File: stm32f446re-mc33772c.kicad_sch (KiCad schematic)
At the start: 43 parts, among them J1 Conn_01x02, J2 USB_B_Micro, J3 Conn_01x03, J4 Conn_01x03, J6 SM06B-GHS-TB, U1 STM32F446RET6, U3 LD1086D2M33TR, U4 AMS1117-3.3, U6 LMR51450SDRRR, U7 SN65HVD232, Y1 16MHz

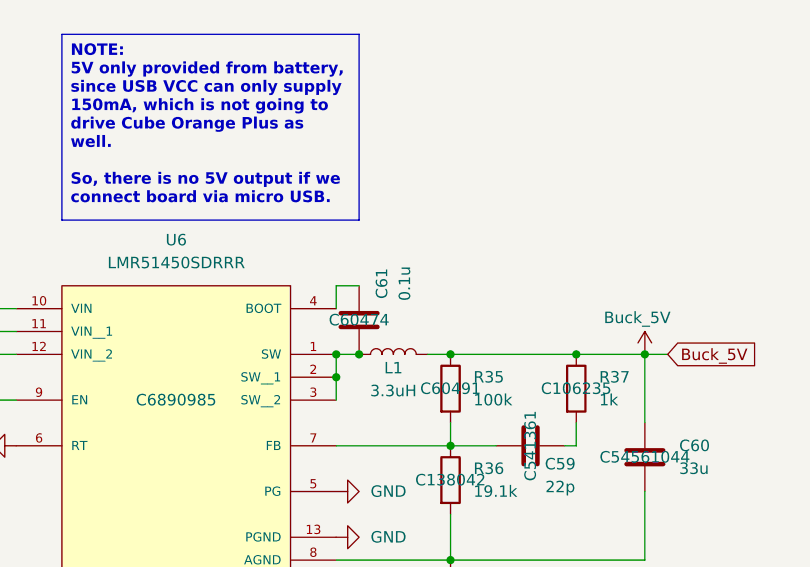
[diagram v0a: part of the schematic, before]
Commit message: export to JLCPCB
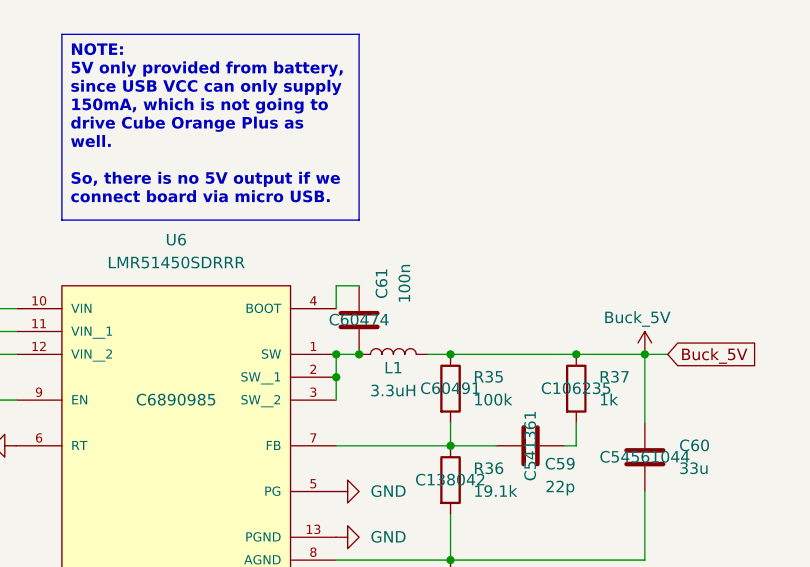
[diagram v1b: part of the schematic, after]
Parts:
- C61: value 0.1u -> 100n
- J1, J3, J4: FT Rotation Offset (none) -> 90
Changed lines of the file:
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@@
 			)
 		)
-		(property "Value" "0.1u"
+		(property "Value" "100n"
 			(at 223.52 122.936 90)
 			(show_name no)
@@
 			)
 		)
+		(property "FT Rotation Offset" "90"
+			(at 148.59 176.53 0)
+			(hide yes)
+			(show_name no)
+			(do_not_autoplace no)
+			(effects
+				(font
+					(size 1.27 1.27)
+				)
+			)
+		)
 		(pin "1"
 		)
@@
 			)
 		)
+		(property "FT Rotation Offset" "90"
+			(at 41.91 97.79 0)
+			(hide yes)
+			(show_name no)
+			(do_not_autoplace no)
+			(effects
+				(font
+					(size 1.27 1.27)
+				)
+			)
+		)
 		(pin "1"
 		)
@@
 			(show_name no)
 			(do_not_autoplace no)
+			(effects
+				(font
+					(size 1.27 1.27)
+				)
+			)
+		)
+		(property "FT Rotation Offset" "90"
+			(at 127 27.94 0)
+			(hide yes)
+			(show_name no)
+			(do_not_autoplace no)

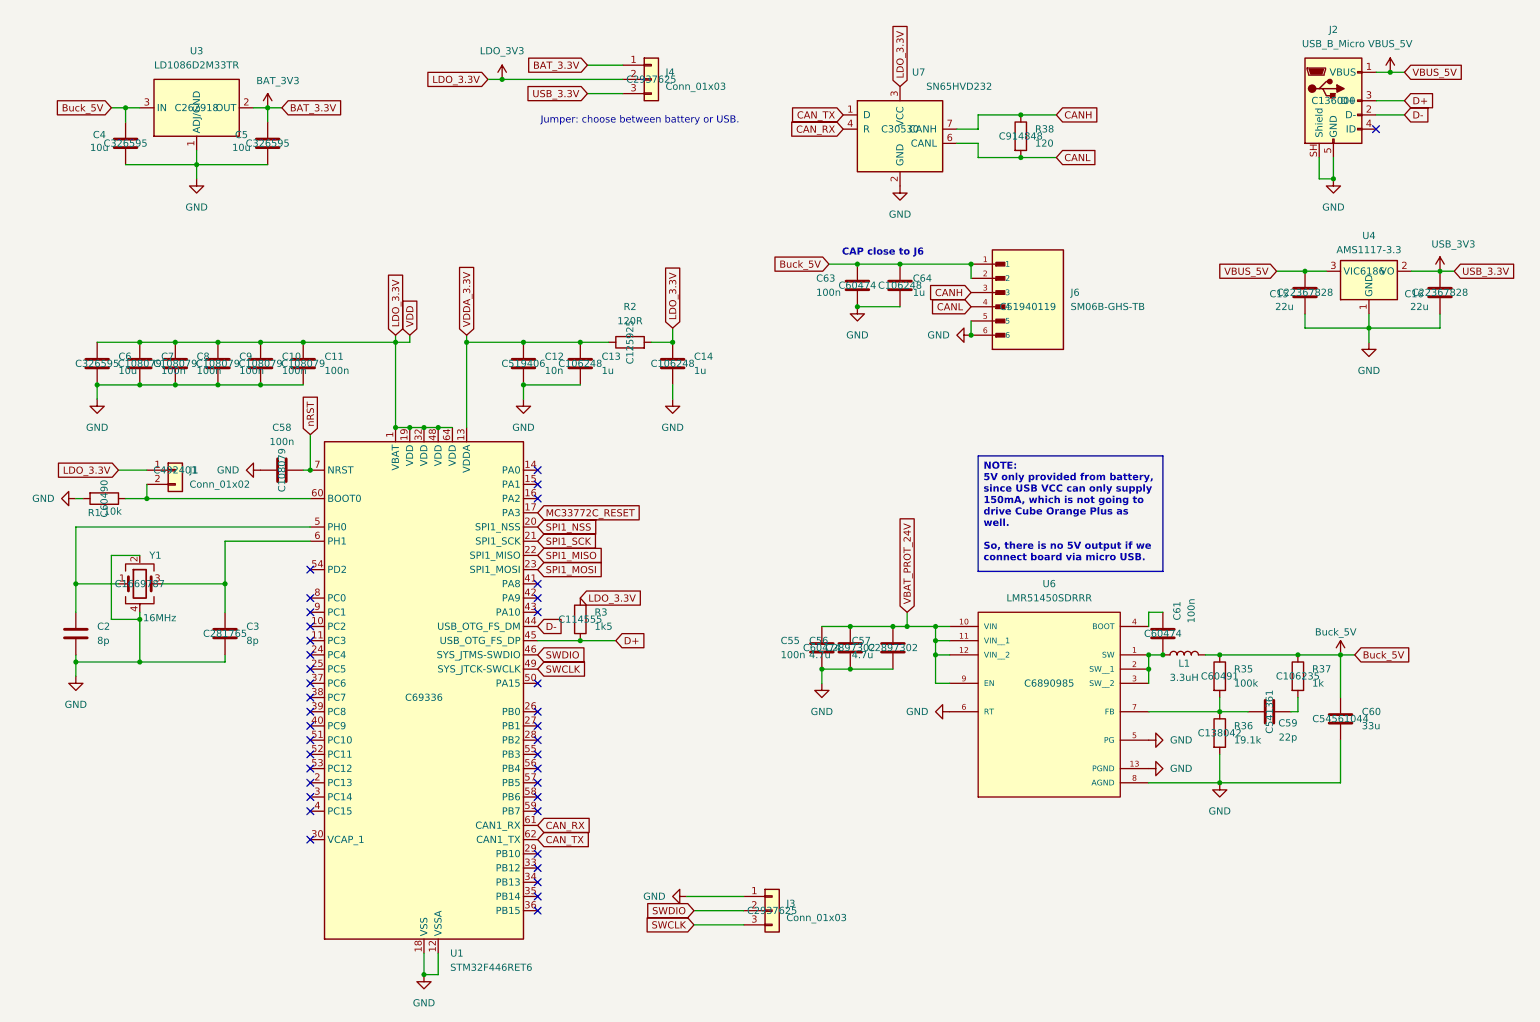
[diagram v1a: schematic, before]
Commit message: for PCBWay
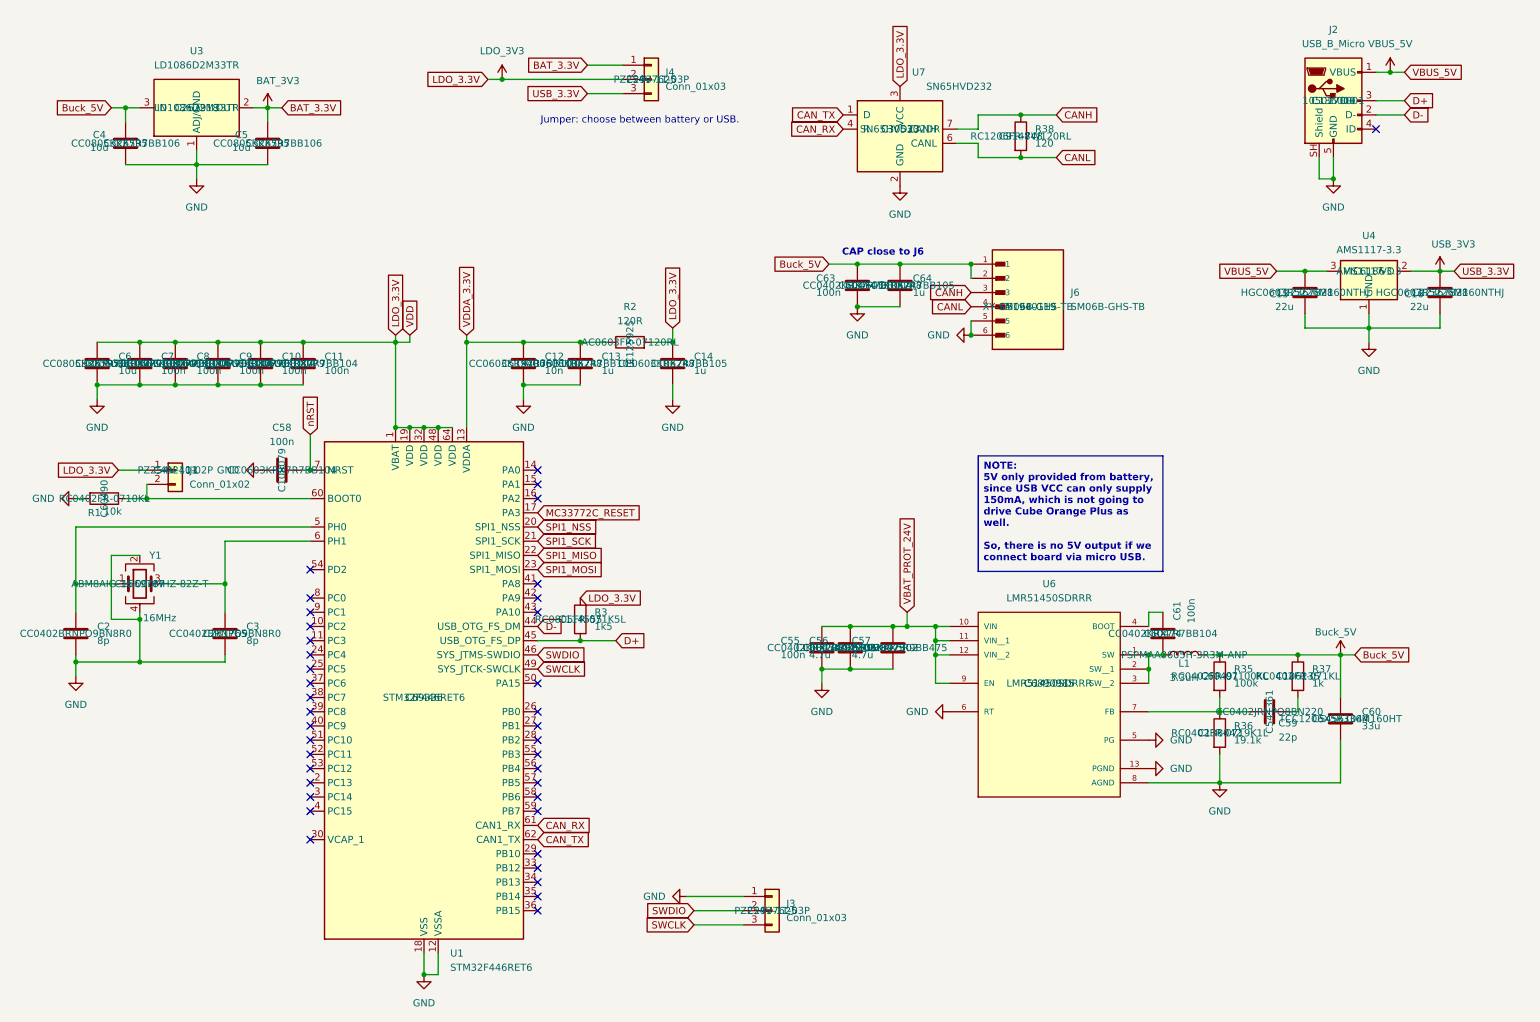
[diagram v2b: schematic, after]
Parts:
- C10, C11, C58, C7, C8, C9: MPN (none) -> CC0603KRX7R7BB104
- C12: MPN (none) -> CC0603KRX7R7BB103
- C13, C14, C64: MPN (none) -> CC0603KRX7R7BB105
- C15, C16: MPN (none) -> HGC0603R5226M160NTHJ
- C2, C3: MPN (none) -> CC0402BRNPO9BN8R0
- C4, C5, C6: MPN (none) -> CC0805KKX7R7BB106
- C55, C61, C63: MPN (none) -> CC0402KRX7R7BB104
- C56, C57: MPN (none) -> CC0805KKX5R9BB475
- C59: MPN (none) -> CC0402JRNPO8BN220
- C60: MPN (none) -> TCC1206X5R336M160HT
- J1: MPN (none) -> PZ254V-11-02P
- J2: MPN (none) -> 1050170001
- J3, J4: MPN (none) -> PZ254V-11-03P
- J6: MPN (none) -> XY-SM06B-GHS-TB
- L1: MPN (none) -> PSPMAA0605H-3R3M-ANP
- R1: MPN (none) -> RC0402FR-0710KL
- R2: MPN (none) -> AC0603FR-07120RL
- R3: MPN (none) -> RC0805FR-071K5L
- R35: MPN (none) -> RC0402FR-07100KL
- R36: MPN (none) -> RC0402FR-0719K1L
- R37: MPN (none) -> RC0402FR-071KL
- R38: MPN (none) -> RC1206FR-7W120RL
- U1: MPN (none) -> STM32F446RET6
- U3: MPN (none) -> LD1086D2M33TR
- U4: MPN (none) -> AMS1117-3.3
- U6: MPN (none) -> LMR51450SDRRR
- U7: MPN (none) -> SN65HVD232DR
- Y1: MPN (none) -> ABM8AIG-16.000MHZ-82Z-T
